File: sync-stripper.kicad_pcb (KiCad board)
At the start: 2 copper layers, 32 x 19 mm, 11 parts, among them J1 5V, J2 SYNC, J3 VIDEO, J4 GND, U1 LM1881

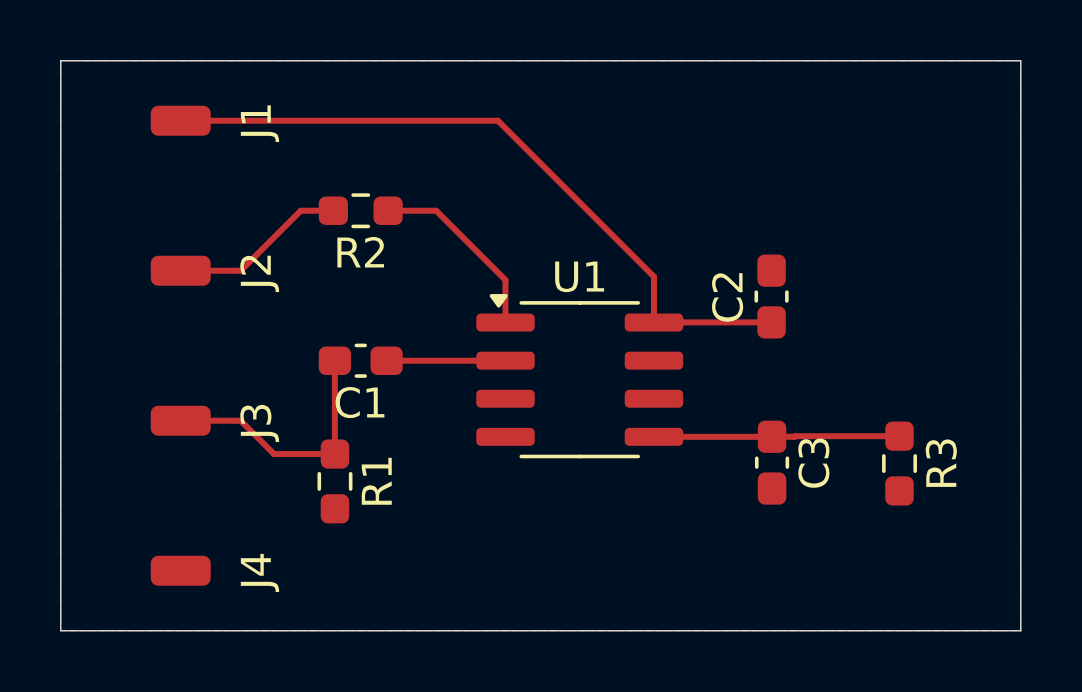
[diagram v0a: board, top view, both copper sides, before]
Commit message: More compact design
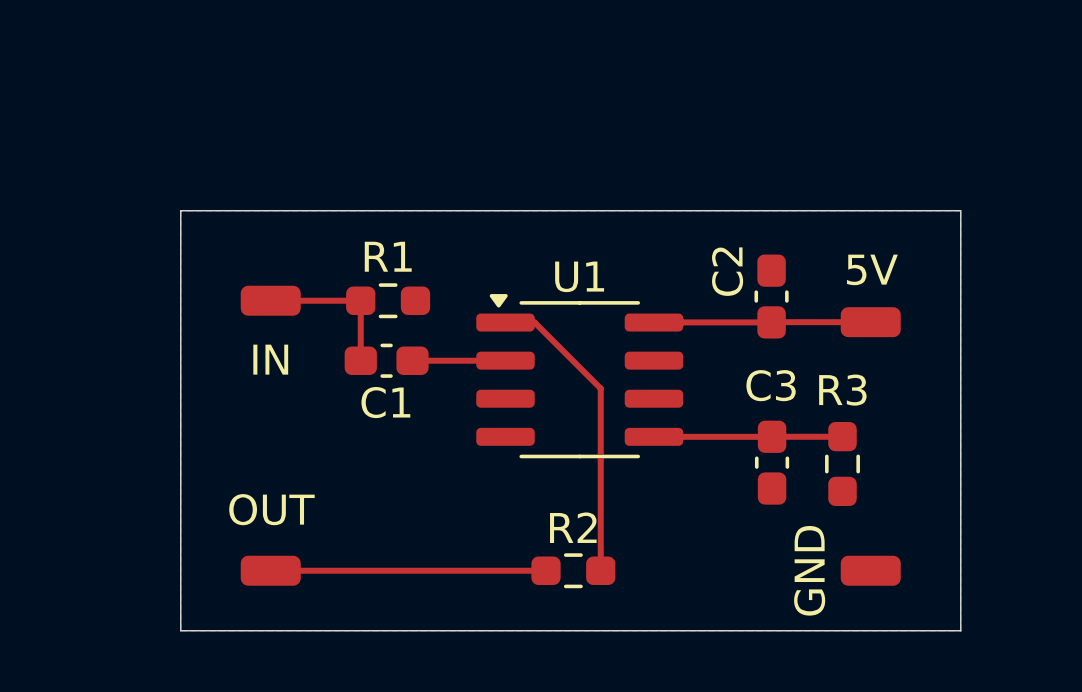
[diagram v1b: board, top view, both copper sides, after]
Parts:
- moved 5V 24.0 mm to (127.0, 88.7), turned to 90 degrees
- moved GND 23.0 mm to (127.0, 97.0)
- moved R2 13.9 mm to (117.1, 97.0)
- moved OUT 10.4 mm to (107.0, 97.0)
- moved R1 6.28 mm to (110.9, 88.0), turned to 0 degrees
- moved IN 5.00 mm to (107.0, 88.0)
- moved R3 1.90 mm to (126.1, 93.4)
- moved C1 0.86 mm to (110.9, 90.0)
- renumbered J1 to 5V, J4 to GND, J3 to IN, J2 to OUT
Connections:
- net SYNC renamed Net-(J2-Pin_1)
- net VIDEO renamed Net-(J3-Pin_1)
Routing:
- net +5V: track 23.4 -> 7.23 mm
- net Net-(U1-CSYNC): track 6.29 -> 10.2 mm
- net Net-(J3-Pin_1): track 8.71 -> 5.00 mm
- net Net-(J2-Pin_1): track 5.92 -> 9.17 mm
- net Net-(U1-BURST): track 8.19 -> 6.29 mm
- net Net-(U1-VIDEO): track 3.96 -> 3.10 mm
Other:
- board size 32 x 19 mm -> 26 x 14 mm
